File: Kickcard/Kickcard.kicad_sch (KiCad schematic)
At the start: 23 parts, among them J1 Conn_Side_Expansion, J2 Conn_01x01_Pin, SW1 SW_DIP_x04, SW2 SW_MEC_5E, SW3 SW_MEC_5E, U1 PAL20L8, U2 SST39SF040, U3 SST39SF040, U4 27C400

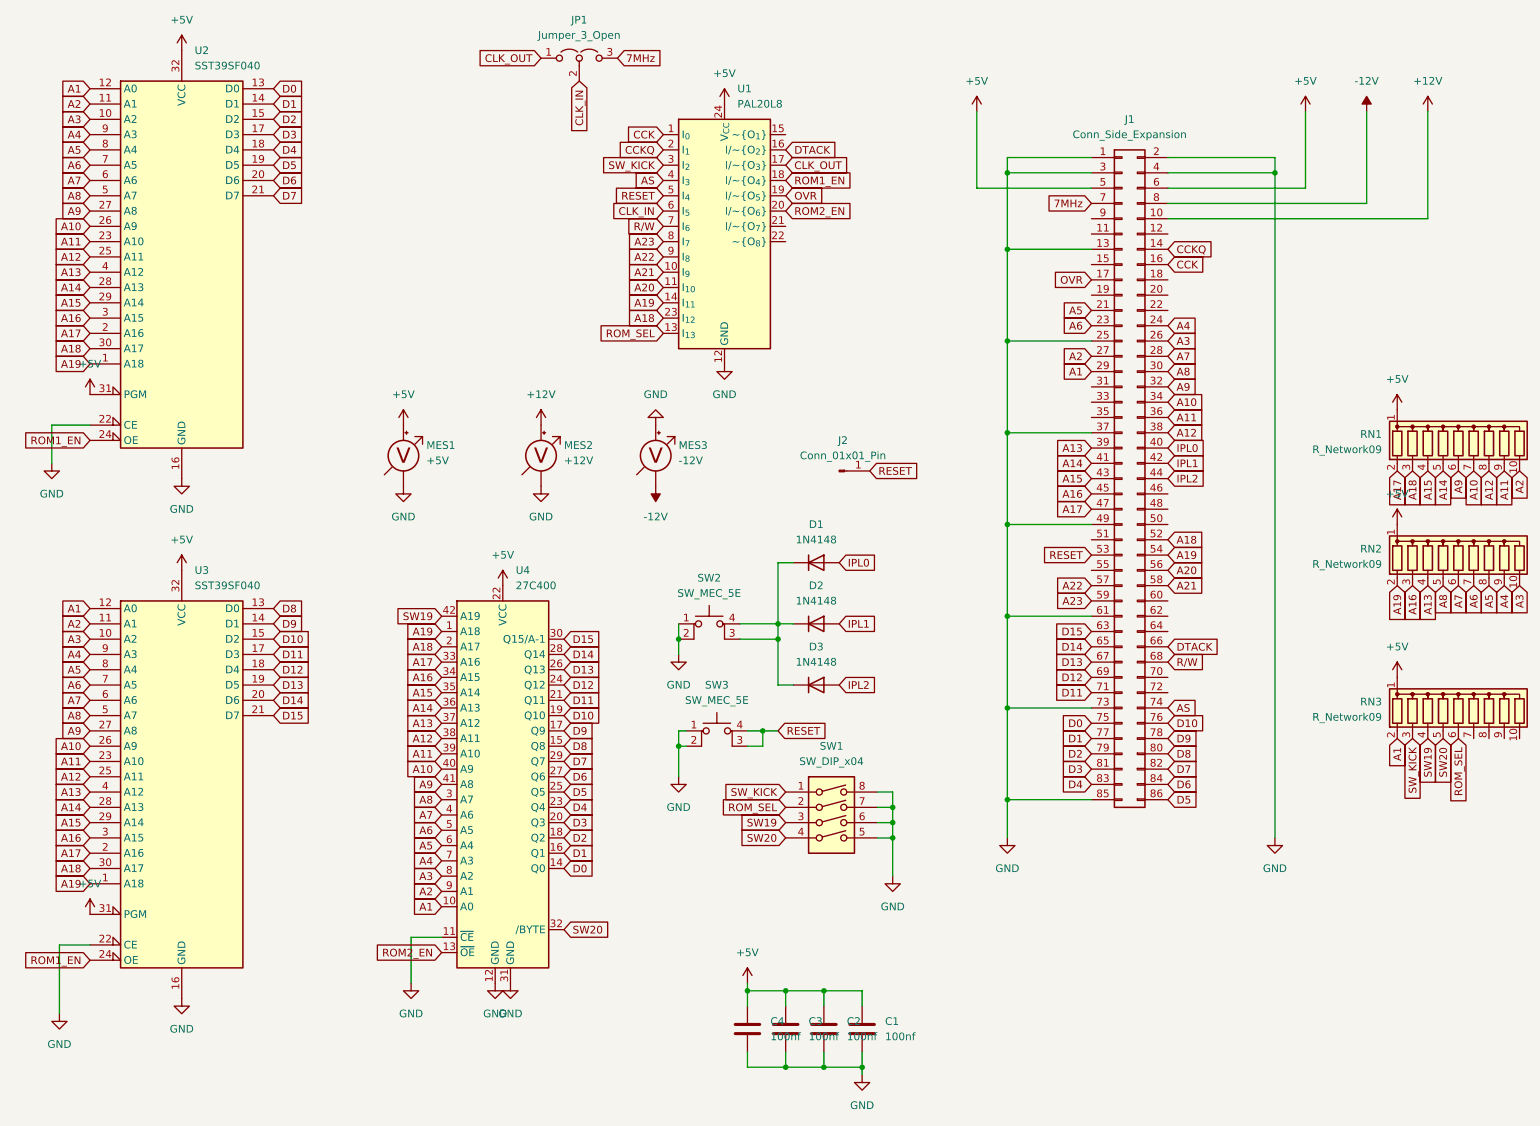
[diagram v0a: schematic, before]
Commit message: added test points
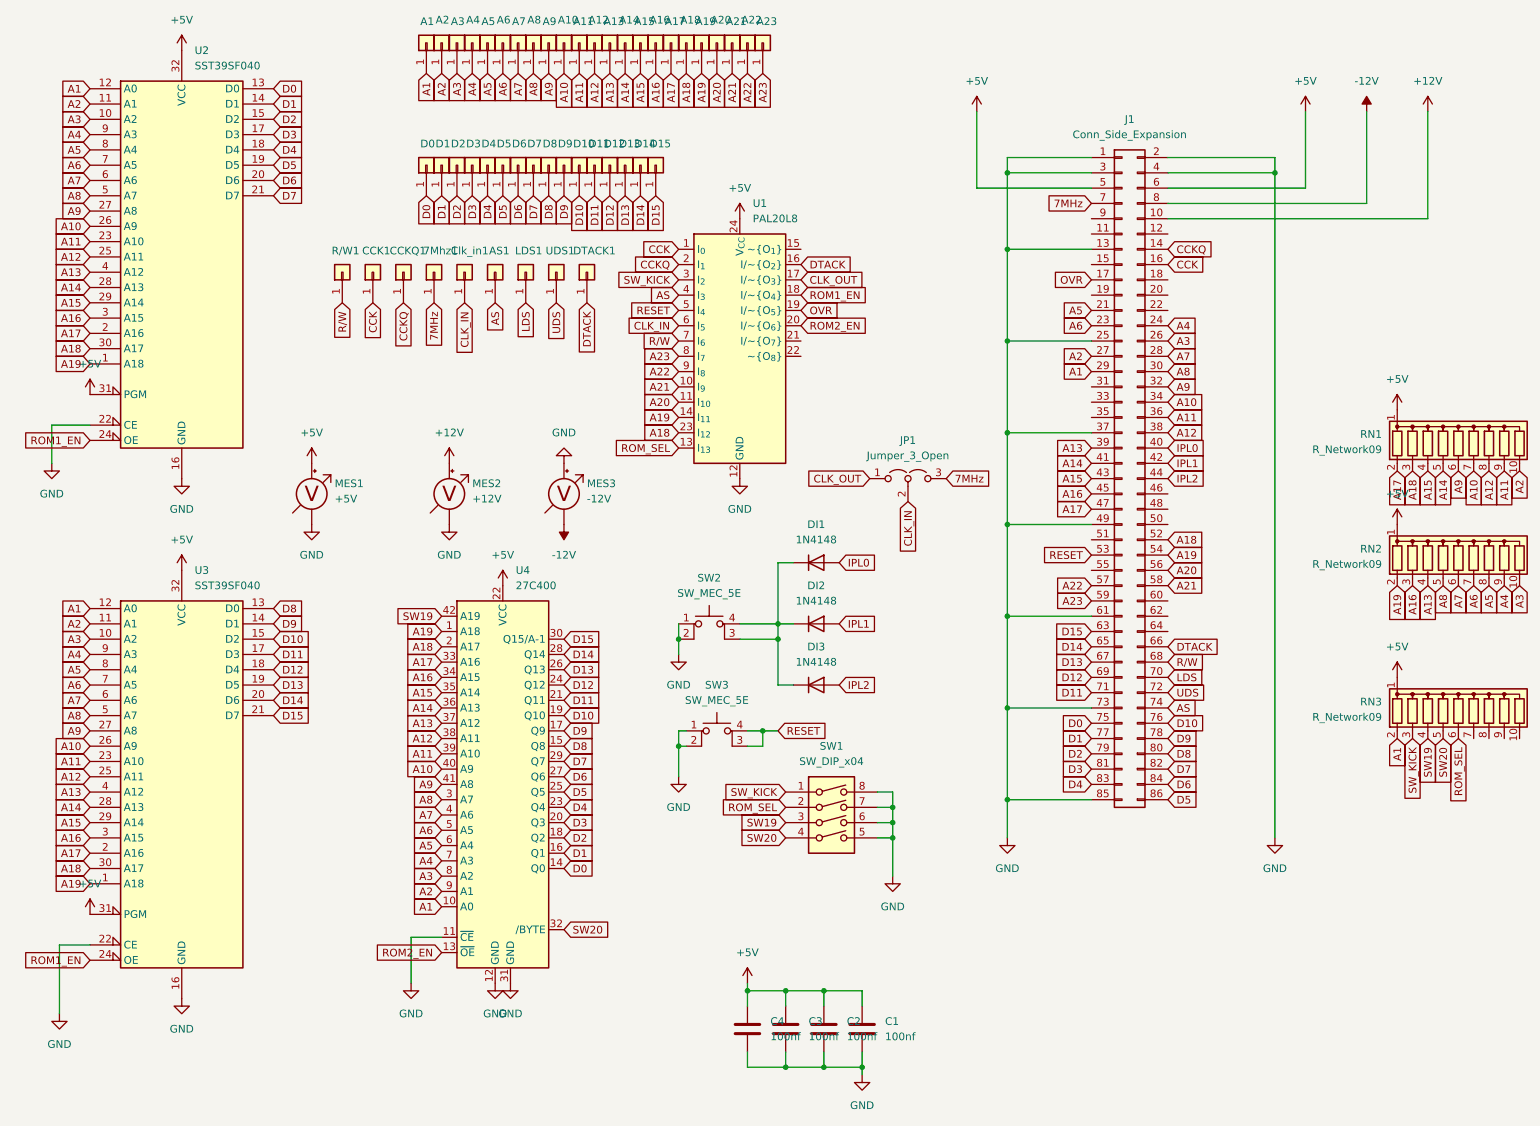
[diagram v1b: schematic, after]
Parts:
- removed J2: Conn_01x01_Pin, Connector_PinHeader_2.54mm:PinHeader_1x01_P2.54mm_Vertical, symbol Connector:Conn_01x01_Pin
- added 7Mhz1, A1, A10, A11, A12, A13, A14, A15, A16, A17, A18, A19, A2, A20, A21, A22, A23, A3, A4, A5, A6, A7, A8, A9, AS1, CCK1, CCKQ1, Clk_in1, D0, D1, D10, D11, D12, D13, D14, D15, D2, D3, D4, D5, D6, D7, D8, D9, DTACK1, LDS1, R/W1, UDS1: Conn_01x01, TestPoint:TestPoint_Pad_D1.0mm, symbol Connector_Generic:Conn_01x01
- renumbered D1 to DI1, D2 to DI2, D3 to DI3
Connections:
- net 7MHz: now also 7Mhz1.1 (Pin_1)
- net A1: now also A1.1 (Pin_1)
- net A10: now also A10.1 (Pin_1)
- net A11: now also A11.1 (Pin_1)
- net A12: now also A12.1 (Pin_1)
- net A13: now also A13.1 (Pin_1)
- net A14: now also A14.1 (Pin_1)
- net A15: now also A15.1 (Pin_1)
- net A16: now also A16.1 (Pin_1)
- net A17: now also A17.1 (Pin_1)
- net A18: now also A18.1 (Pin_1)
- net A19: now also A19.1 (Pin_1)
- net A2: now also A2.1 (Pin_1)
- net A20: now also A20.1 (Pin_1)
- net A21: now also A21.1 (Pin_1)
- net A22: now also A22.1 (Pin_1)
- net A23: now also A23.1 (Pin_1)
- net A3: now also A3.1 (Pin_1)
- net A4: now also A4.1 (Pin_1)
- net A5: now also A5.1 (Pin_1)
- net A6: now also A6.1 (Pin_1)
- net A7: now also A7.1 (Pin_1)
- net A8: now also A8.1 (Pin_1)
- net A9: now also A9.1 (Pin_1)
- net AS: now also AS1.1 (Pin_1)
- net CCK: now also CCK1.1 (Pin_1)
- net CCKQ: now also CCKQ1.1 (Pin_1)
- net CLK_IN: now also Clk_in1.1 (Pin_1)
- net D0: now also D0.1 (Pin_1)
- net D1: now also D1.1 (Pin_1)
- net D10: now also D10.1 (Pin_1)
- net D11: now also D11.1 (Pin_1)
- net D12: now also D12.1 (Pin_1)
- net D13: now also D13.1 (Pin_1)
- net D14: now also D14.1 (Pin_1)
- net D15: now also D15.1 (Pin_1)
- net D2: now also D2.1 (Pin_1)
- net D3: now also D3.1 (Pin_1)
- net D4: now also D4.1 (Pin_1)
- net D5: now also D5.1 (Pin_1)
- net D6: now also D6.1 (Pin_1)
- net D7: now also D7.1 (Pin_1)
- net D8: now also D8.1 (Pin_1)
- net D9: now also D9.1 (Pin_1)
- net DTACK: now also DTACK1.1 (Pin_1)
- net R/W: now also R/W1.1 (Pin_1)
- net LDS: now reaches J1.70 (_LDS)
- net LDS: now also LDS1.1 (Pin_1)
- net UDS: now reaches J1.72 (_UDS)
- net UDS: now also UDS1.1 (Pin_1)
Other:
- moved on the sheet: JP1, MES1, MES2, MES3, U1
